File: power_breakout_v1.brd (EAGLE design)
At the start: 160 x 100 mm, 4 parts, among them IC1 LP2950CZ-3.3

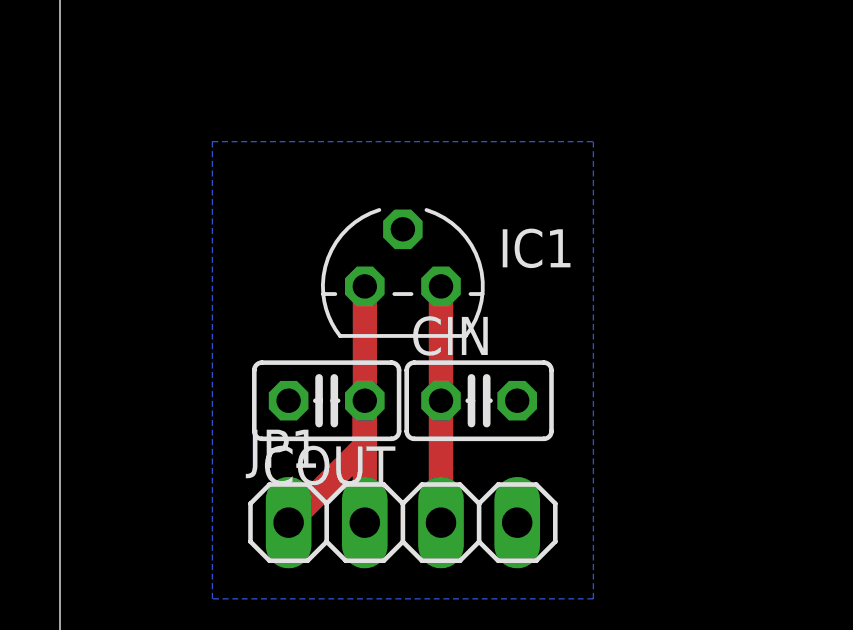
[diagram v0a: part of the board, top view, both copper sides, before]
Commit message: pcbWayCheckPassed
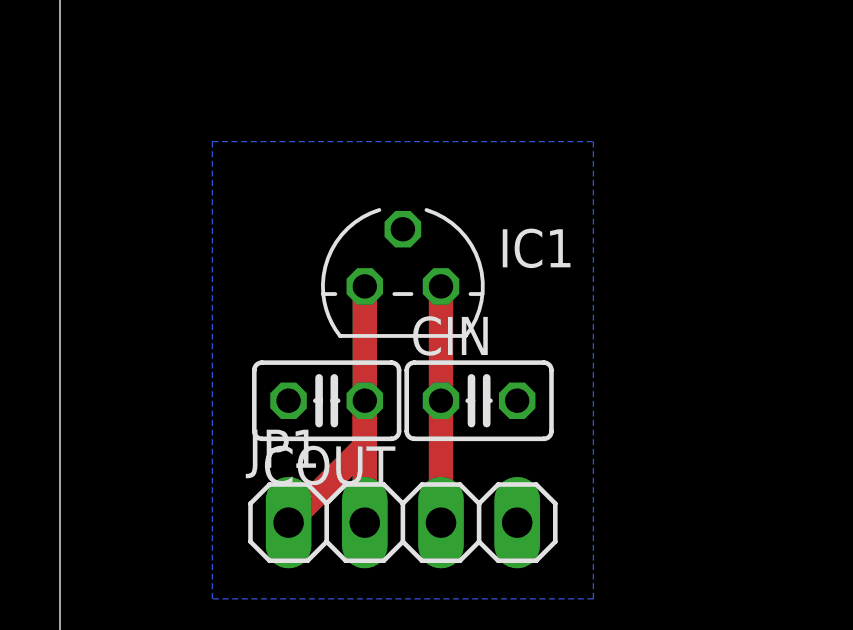
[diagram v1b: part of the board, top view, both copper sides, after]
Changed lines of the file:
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@@
 </class>
 </classes>
-<designrules name="default">
+<designrules name="PCBWay_2layer">
 <description language="de">&lt;b&gt;EAGLE Design Rules&lt;/b&gt;
 &lt;p&gt;
@@
 <param name="mdPadVia" value="6mil"/>
 <param name="mdViaVia" value="6mil"/>
-<param name="mdSmdPad" value="6mil"/>
-<param name="mdSmdVia" value="6mil"/>
-<param name="mdSmdSmd" value="6mil"/>
-<param name="mdViaViaSameLayer" value="6mil"/>
+<param name="mdSmdPad" value="4mil"/>
+<param name="mdSmdVia" value="4mil"/>
+<param name="mdSmdSmd" value="4mil"/>
+<param name="mdViaViaSameLayer" value="8mil"/>
 <param name="mnLayersViaInSmd" value="2"/>
-<param name="mdCopperDimension" value="40mil"/>
+<param name="mdCopperDimension" value="10mil"/>
 <param name="mdDrill" value="6mil"/>
 <param name="mdSmdStop" value="0mil"/>
 <param name="msWidth" value="6mil"/>
-<param name="msDrill" value="0.35mm"/>
-<param name="msMicroVia" value="9.99mm"/>
+<param name="msDrill" value="0.3mm"/>
+<param name="msMicroVia" value="0.3mm"/>
 <param name="msBlindViaRatio" value="0.5"/>
 <param name="rvPadTop" value="0.25"/>
@@
 <param name="rvMicroViaOuter" value="0.25"/>
 <param name="rvMicroViaInner" value="0.25"/>
-<param name="rlMinPadTop" value="10mil"/>
+<param name="rlMinPadTop" value="6mil"/>
 <param name="rlMaxPadTop" value="20mil"/>
-<param name="rlMinPadInner" value="10mil"/>
+<param name="rlMinPadInner" value="6mil"/>
 <param name="rlMaxPadInner" value="20mil"/>
-<param name="rlMinPadBottom" value="10mil"/>
+<param name="rlMinPadBottom" value="6mil"/>
 <param name="rlMaxPadBottom" value="20mil"/>
-<param name="rlMinViaOuter" value="8mil"/>
+<param name="rlMinViaOuter" value="6mil"/>
 <param name="rlMaxViaOuter" value="20mil"/>
-<param name="rlMinViaInner" value="8mil"/>
+<param name="rlMinViaInner" value="6mil"/>
 <param name="rlMaxViaInner" value="20mil"/>
-<param name="rlMinMicroViaOuter" value="4mil"/>
+<param name="rlMinMicroViaOuter" value="6mil"/>
 <param name="rlMaxMicroViaOuter" value="20mil"/>
-<param name="rlMinMicroViaInner" value="4mil"/>
+<param name="rlMinMicroViaInner" value="6mil"/>
 <param name="rlMaxMicroViaInner" value="20mil"/>
 <param name="psTop" value="-1"/>
@@
 <param name="mlMinCreamFrame" value="0mil"/>
 <param name="mlMaxCreamFrame" value="0mil"/>
-<param name="mlViaStopLimit" value="0mil"/>
+<param name="mlViaStopLimit" value="0.8mm"/>
 <param name="srRoundness" value="0"/>
 <param name="srMinRoundness" value="0mil"/>
@@
 <param name="slThermalIsolate" value="10mil"/>
 <param name="slThermalsForVias" value="0"/>
-<param name="dpMaxLengthDifference" value="10mm"/>
+<param name="dpMaxLengthDifference" value="1mm"/>
 <param name="dpGapFactor" value="2.5"/>
 <param name="checkAngle" value="0"/>
